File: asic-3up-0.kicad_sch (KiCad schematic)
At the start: 66 parts, among them J12 Conn_01x01, J13 Conn_01x01, J18 Conn_01x01, J3 Conn_01x01, J4 Conn_01x01, U28 MCP1824T-1202E/OT, U29 MCP1824T-1202E/OT, U30 MCP1824T-1202E/OT, U32 MCP1824T-0802E, U42 MCP1824T-0802E, U43 MCP1824T-0802E, U45 BM1362AC_MODE1, U46 BM1362AC_MODE0, U47 BM1362AC_MODE1

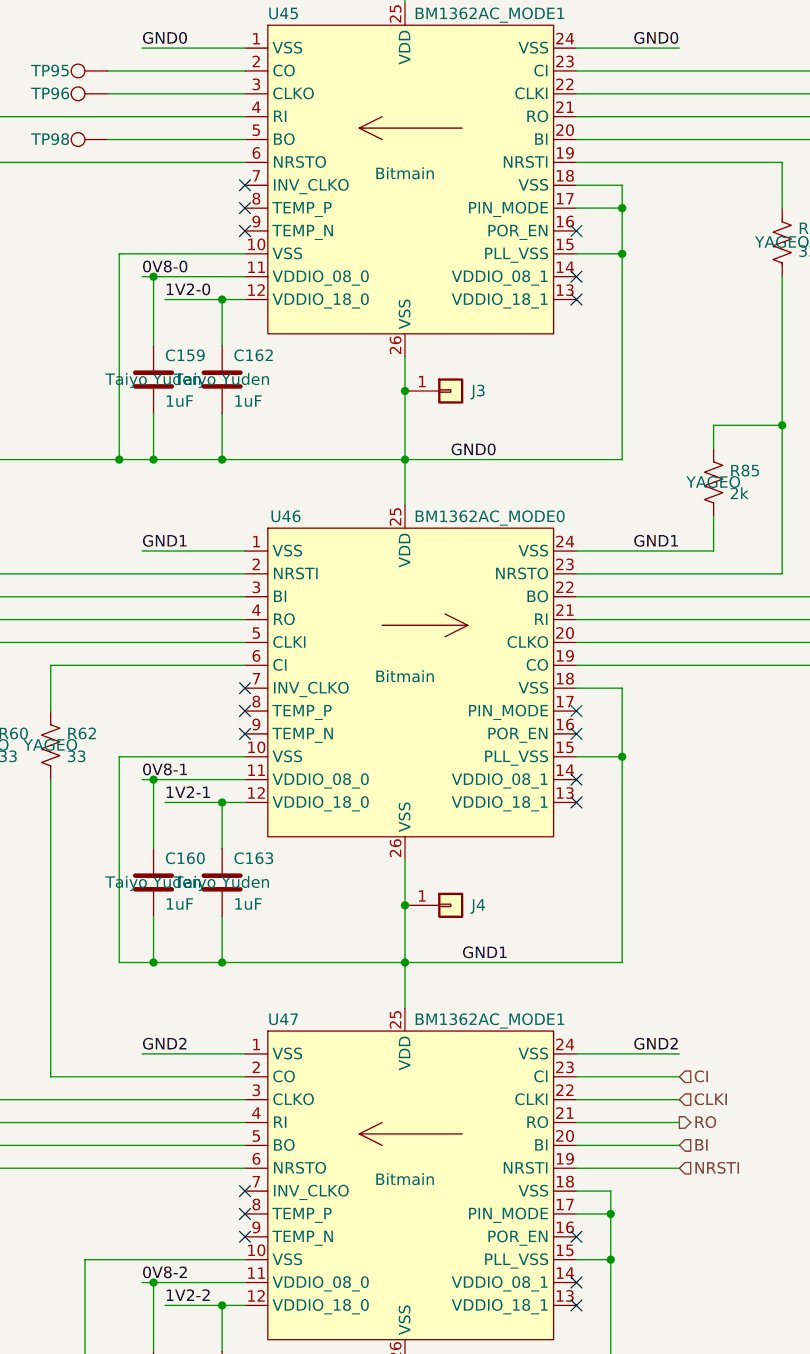
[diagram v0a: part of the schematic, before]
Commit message: missed a few
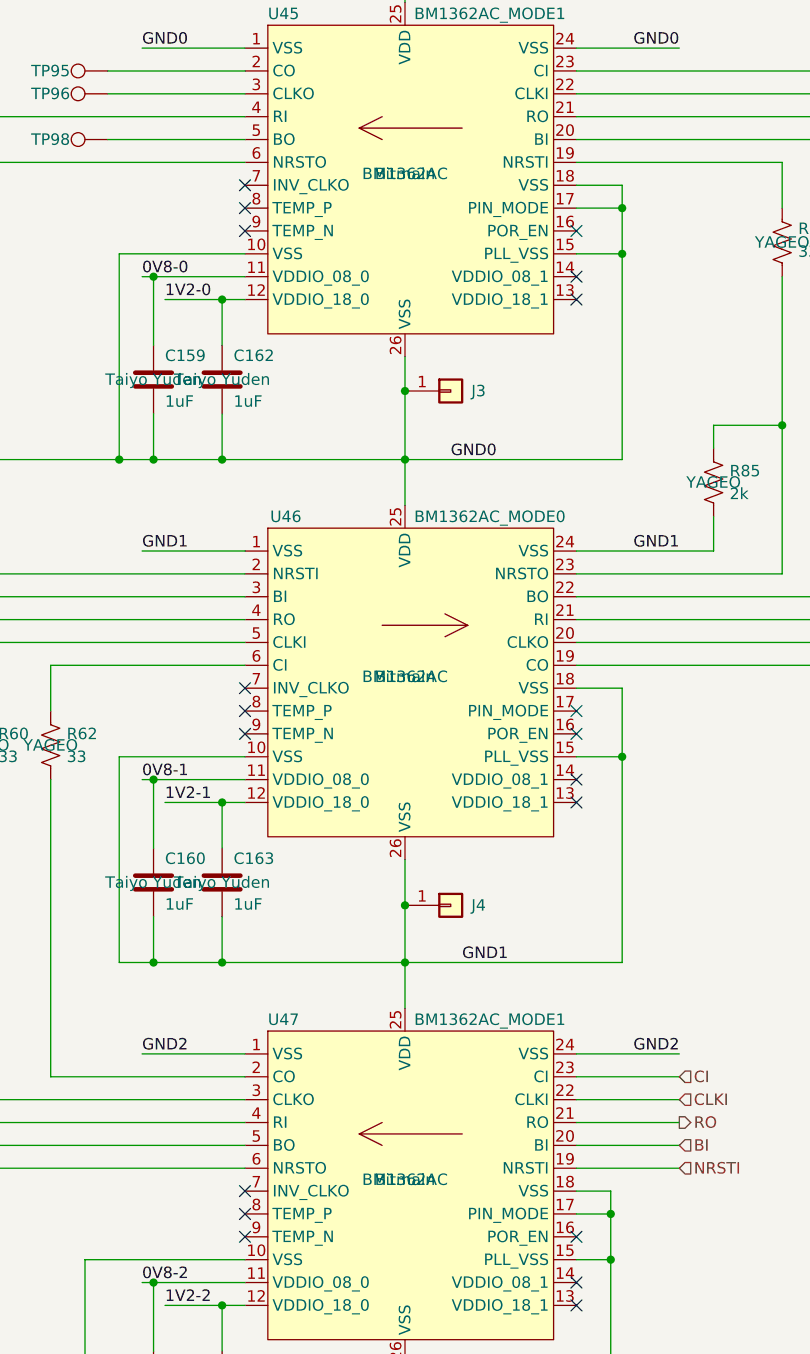
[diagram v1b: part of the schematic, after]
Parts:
- U45, U46, U47: PARTNO (none) -> BM1362AC
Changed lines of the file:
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@@
+			)
+		)
+		(property "PARTNO" "BM1362AC"
+			(at 248.92 78.74 0)
+			(effects
+				(font
+					(size 1.27 1.27)
+				)
 			)
 		)
@@
 			)
 		)
+		(property "PARTNO" "BM1362AC"
+			(at 248.92 134.62 0)
+			(effects
+				(font
+					(size 1.27 1.27)
+				)
+			)
+		)
 		(pin "10"
 		)
@@
 			(at 248.92 190.5 0)
 			(effects
+				(font
+					(size 1.27 1.27)
+				)
+			)
+		)
+		(property "PARTNO" "BM1362AC"
+			(at 248.92 190.5 0)
+			(effects

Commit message: fixed wrong part number
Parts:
- R64: PARTNO RC0402FR-072KL -> RC0402FR-071KL
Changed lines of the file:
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@@
 			)
 		)
-		(property "PARTNO" "RC0402FR-072KL"
+		(property "PARTNO" "RC0402FR-071KL"
 			(at 195.58 66.04 0)
 			(effects

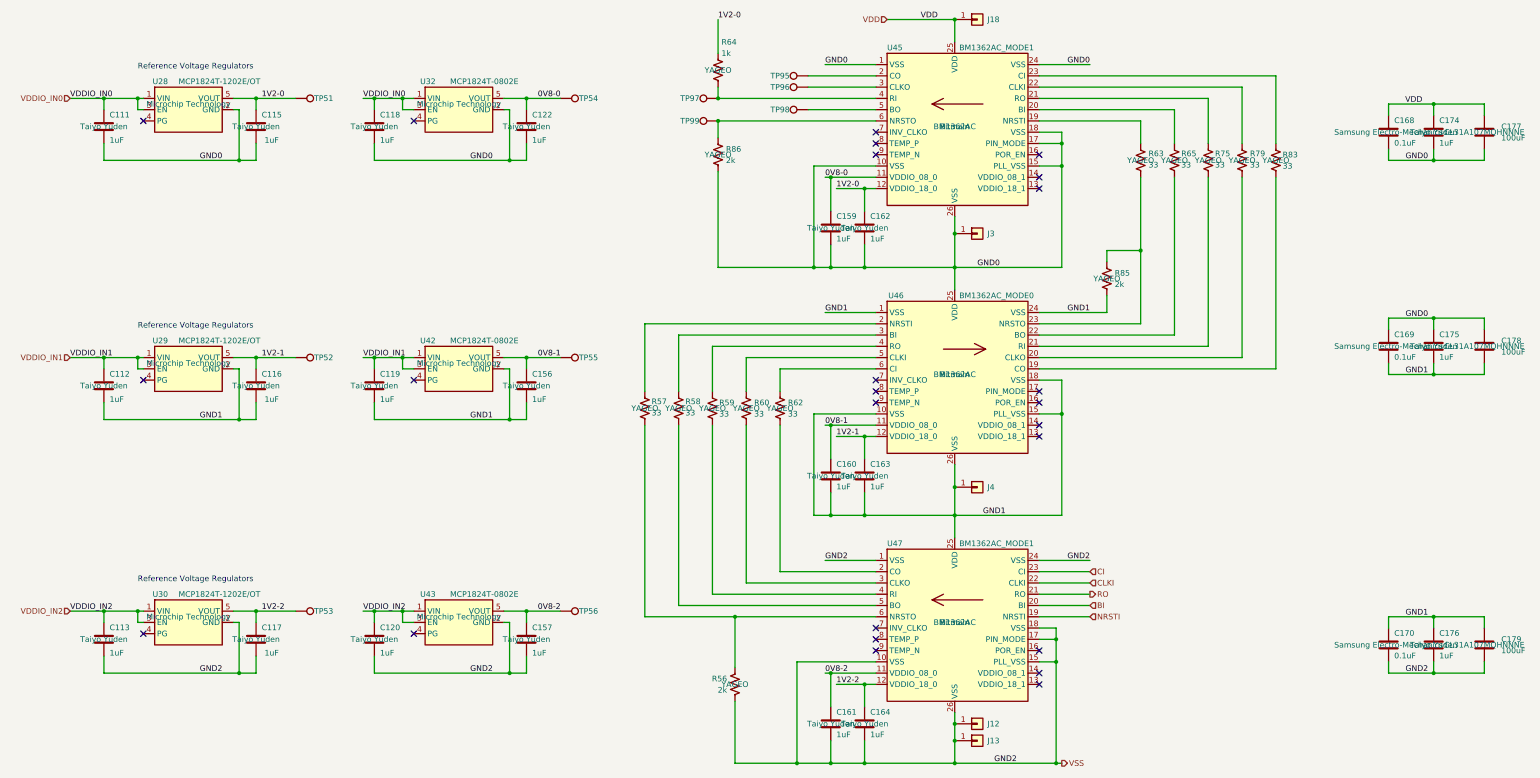
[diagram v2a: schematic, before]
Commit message: Revert "Merge commit '7c9b4c648e8c0cd5eb9ee29b12963992edc9d4fe' into v4"
This reverts commit 16575a5f433ae2a288f6a827ad209afb5e5f3437, reversing
changes made to e5a5abad8ce065f31a2bf126cd7235584780cb09.
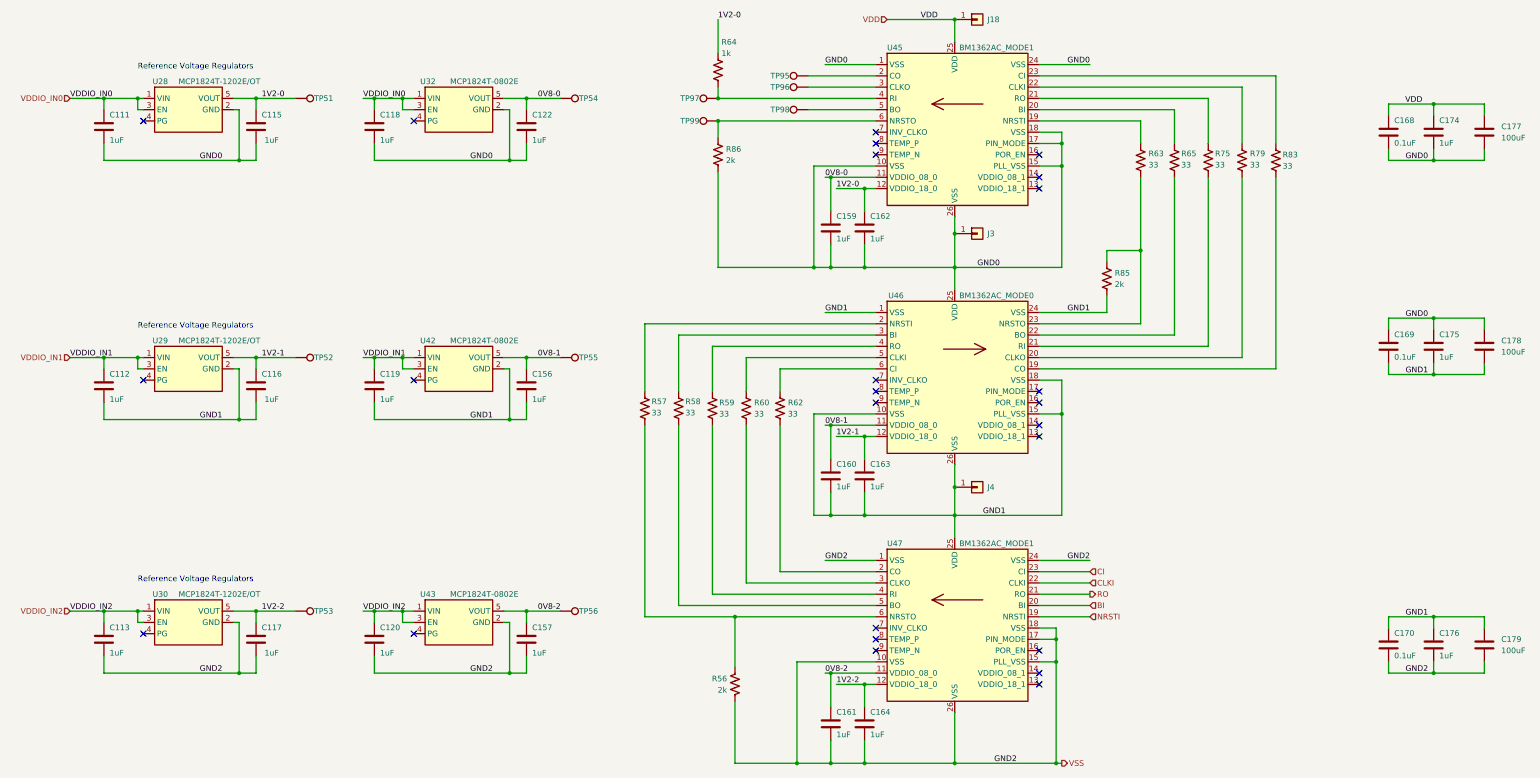
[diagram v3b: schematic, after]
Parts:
- removed J12: Conn_01x01, emberone:14x9_powertab_L, symbol Connector_Generic:Conn_01x01
- removed J13: Conn_01x01, emberone:14x9_powertab_R, symbol Connector_Generic:Conn_01x01
- C111, C112, C113, C115, C116, C117, C118, C119, C120, C122, C156, C157, C159, C160, C161, C162, C163, C164, C174, C175, C176: Manufacturer Taiyo Yuden -> (none)
- C168, C169, C170: DK 1276-1234-1-ND -> 478-KGM05AR71C104KHCT-ND; Manufacturer Samsung Electro-Mechanics -> (none); PARTNO CL05A104KO5NNNC -> KGM05AR71C104KH
- C177, C178, C179: Manufacturer CL31A107MQHNNNE -> (none)
- J18, J3, J4: now in the parts list
- R56, R57, R58, R59, R60, R62, R63, R65, R75, R79, R83, R85, R86: Manufacturer YAGEO -> (none)
- R64: Manufacturer YAGEO -> (none); PARTNO RC0402FR-071KL -> RC0402FR-072KL
- U28, U29, U30: ALT1 (none) -> LDK120M12R; Manufacturer Microchip Technology -> (none)
- U32, U42, U43: ALT1 (none) -> LDK120M08R; Manufacturer Microchip Technology -> (none)
- U45, U46, U47: Manufacturer Bitmain -> (none); PARTNO BM1362AC -> (none)
